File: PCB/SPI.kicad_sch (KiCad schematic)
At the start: 21 parts, among them J3 Trackpad, J4 OLED_Breakout, J6 SSD1351, U4 PMW3360DM-T2QU

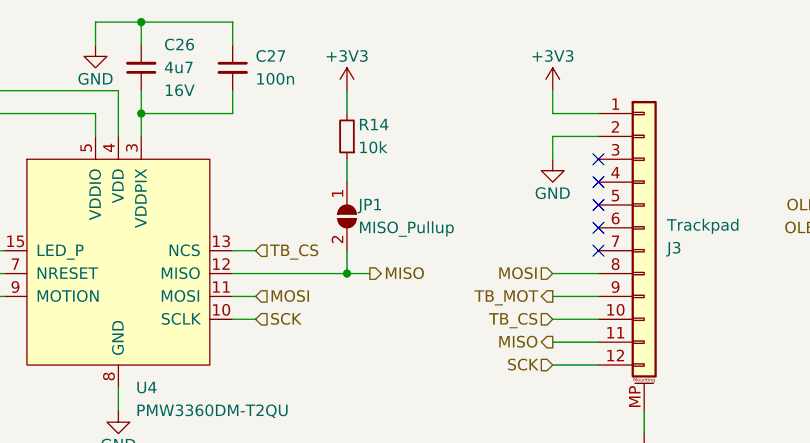
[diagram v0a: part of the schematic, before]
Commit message: 05/05/2023 update.
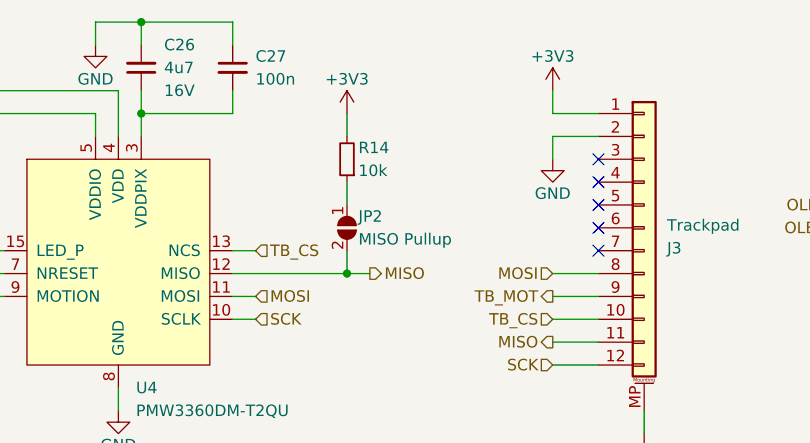
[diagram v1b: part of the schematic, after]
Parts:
- removed D57 (x2): 1N4148, Honeydew:D_SOD-323, symbol Device:D_Small
- removed JP1: MISO_Pullup, Jumper:SolderJumper-2_P1.3mm_Open_Pad1.0x1.5mm, symbol Jumper:SolderJumper_2_Open
- added D57 (x2): 1N4148, Honeydew:D_SOD-323, symbol Device:D_Small
- added JP2: MISO Pullup, Honeydew:SolderJumper-2_P1.2mm_Open_Pad1.0x1.0mm, symbol Honeydew:SolderJumper_2_Open
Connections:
- net GND: now also D57.1 (K)
- net MISO: now also JP2.2 (B)
- net at R14.1: now also JP2.1 (A)
- net at R29.1: now also D57.2 (A)
- new net: D57.1 (K), D57.2 (A)
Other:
- moved on the sheet: R14
